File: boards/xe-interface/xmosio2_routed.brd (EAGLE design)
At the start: 116.8 x 55.2 mm, 105 parts, among them IC1 IDTQS3245QSOP20, IC2 IDTQS3245QSOP20, IC3 IDTQS3245QSOP20, IC4 IDTQS3245QSOP20, IC5 IDTQS3245QSOP20, U1 24 MHz Osc. (F535L-24), U2 USD-SOCKETNEW, X1 0446200002

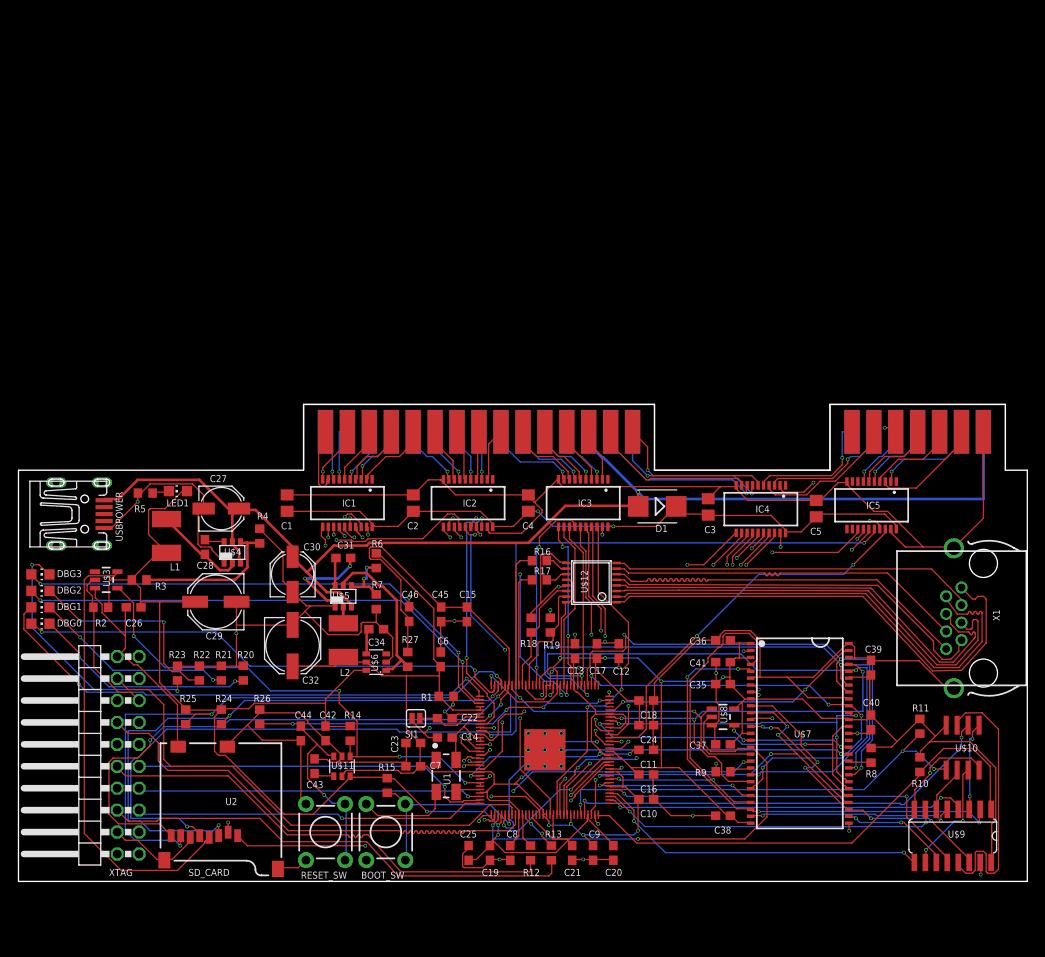
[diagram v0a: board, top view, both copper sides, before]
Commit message: Latest board (routed and unrolled)
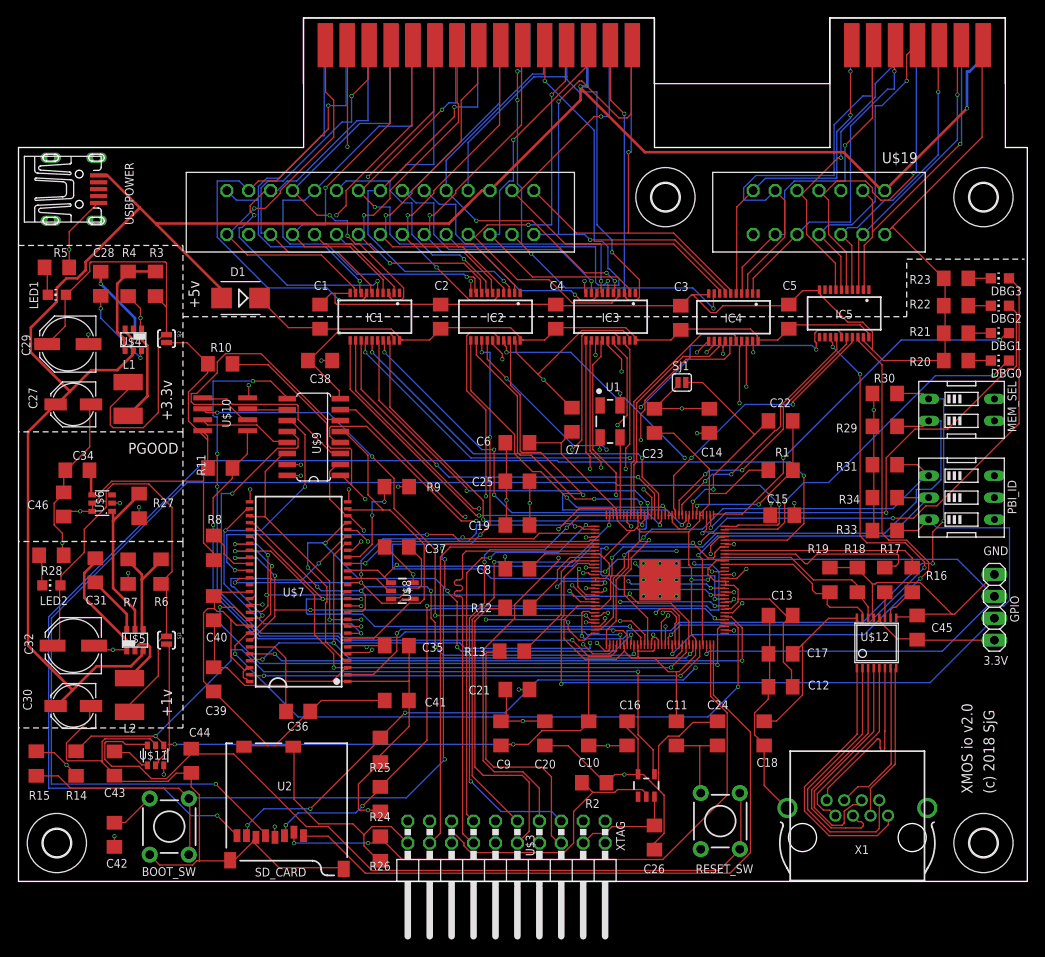
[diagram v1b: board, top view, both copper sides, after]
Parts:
- added GPIO: (no value), pinhead:1X04
- added H1, H2, H3, H4: MOUNT-HOLE3.2, holes:3,2
- added LED2: ok33, led:CHIP-LED0805
- added MEM_SEL: (no value), special:EDG-02
- added PBI_ID: (no value), special:EDG-03
- added R28: 47R, rcl:R1206
- added R29, R30, R31, R33, R34: 10K, rcl:R1206
- added SJ2, SJ3: SOLDERJUMPERNO, SparkFun:SJ_2S-NO
- added U$19: XE_SLOT, pbxl:XE_SLOT
- C1, C2, C3, C4, C5: device rcl:C0805 -> rcl:C1206
- C10, C11, C12, C13, C14, C15, C16, C17, C18, C19, C20, C21, C22, C23, C24, C25, C26, C28, C31, C34, C35, C36, C37, C38, C39, C40, C41, C42, C43, C44, C45, C46, C6, C7, C8, C9: device rcl:C0603 -> rcl:C1206
- R1, R10, R11, R12, R13, R14, R15, R16, R17, R18, R19, R2, R20, R21, R22, R23, R24, R25, R26, R27, R3, R4, R5, R6, R7, R8, R9: device rcl:R0603 -> rcl:R1206
- moved DBG3 116.3 mm to (113.7, 69.8), turned to 90 degrees
- moved DBG2 115.9 mm to (113.7, 66.7), turned to 90 degrees
- moved DBG1 115.6 mm to (113.7, 63.5), turned to 90 degrees
- moved DBG0 115.2 mm to (113.7, 60.3), turned to 90 degrees
- moved R23 101.1 mm to (108.6, 69.8), turned to 180 degrees
- moved R22 97.4 mm to (108.6, 66.7), turned to 180 degrees
- moved R21 93.8 mm to (108.6, 63.5), turned to 180 degrees
- moved U$10 93.7 mm to (23.9, 54.1), turned to 90 degrees
- moved R10 93.4 mm to (23.4, 59.9), turned to 0 degrees
- moved R20 90.1 mm to (108.6, 60.3), turned to 180 degrees
- moved U$9 87.2 mm to (34.2, 51.5), turned to 90 degrees
- moved R11 86.4 mm to (23.4, 47.9), turned to 0 degrees
- moved R8 79.8 mm to (22.6, 38.6), turned to 90 degrees
- moved C40 77.3 mm to (22.6, 31.7), turned to 90 degrees
- moved C39 76.1 mm to (22.6, 23.4), turned to 270 degrees
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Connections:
- new net N$30: C29.+, L1.1, LED1.A, R3.2, SJ2.1
- new net N$31: LED2.C, R28.2
- new net N$32: C32.+, L2.1, LED2.A, R6.2, SJ3.1
- new net N$34: MEM_SEL.2, R29.1, U$2.25
- new net N$35: MEM_SEL.1, R30.2, U$2.26
- new net N$36: GPIO.3, U$2.12
- new net N$37: GPIO.2, U$2.14
- new net PBI0: PBI_ID.1, R31.2, U$2.33
- new net PBI1: PBI_ID.2, R34.2, U$2.61
- new net PBI2: PBI_ID.3, R33.2, U$2.62
- net +5V: now also U$19.26, U$19.44
- net B1: now also U$19.1
- net B10: now also U$19.11
- net B11: now also U$19.12
- net B12: now also U$19.13
- net B13: now also U$19.14
- net B14: now also U$19.15
- net B15: now also U$19.16
- net B16: now also U$19.17
- net B17: now also U$19.18
- net B18: now also U$19.19
- net B19: now also U$19.20
- net B2: now also U$19.2
- net B20: now also U$19.21
- net B21: now also U$19.22
- net B22: now also U$19.23
- net B23: now also U$19.24
- net B24: now also U$19.25
- net B25: now also U$19.27
- net B26: now also U$19.28
- net B27: now also U$19.29
- net B28: now also U$19.30
- net B29: now also U$19.32
- net B3: now also U$19.4
- net B30: now also U$19.33
- net B31: now also U$19.34
- net B32: now also U$19.35
- net B33: now also U$19.36
- net B34: now also U$19.37
- net B35: now also U$19.38
- net B36: now also U$19.39
- net B37: now also U$19.41
- net B38: now also U$19.42
- net B4: now also U$19.5
- net B5: now also U$19.6
- net B6: now also U$19.7
- net B7: now also U$19.8
- net B8: now also U$19.9
- net B9: now also U$19.10
- net GND: now also GPIO.1, R28.1, R29.2, R30.1, R31.1, R33.1, R34.1, U$19.3, U$19.43
- net VCCINT: now also SJ3.2; no longer C32.+, L2.1, R6.2, U$6.5
- net VCCIO: now also GPIO.4, MEM_SEL.3, MEM_SEL.4, PBI_ID.4, PBI_ID.5, PBI_ID.6, SJ2.2, U$6.5; no longer C29.+, L1.1, LED1.A, R3.2
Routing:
- net VCCIO: track 456.0 -> 256.4 mm, vias 10 -> 29
- net +5V: track 145.0 -> 238.6 mm, vias 1 -> 2
- net SDC_D1: track 64.5 -> 155.1 mm
- net GND: track 464.6 -> 551.5 mm, vias 32 -> 37
- net SDC_CLK: track 69.7 -> 147.2 mm
- net N$33: track 23.3 -> 99.8 mm, vias 1 -> 3
- net N$21: track 22.1 -> 96.7 mm, vias 1 -> 0
- net N$35: track 0.00 -> 74.3 mm, vias 0 -> 3
- net N$36: track 0.00 -> 70.2 mm, vias 0 -> 1
- net N$34: track 0.00 -> 62.0 mm, vias 0 -> 1
- net PBI2: track 0.00 -> 61.1 mm, vias 0 -> 1
- net N$32: track 0.00 -> 56.3 mm
- net VCCINT: track 174.3 -> 228.8 mm, vias 10 -> 4
- net PBI0: track 0.00 -> 54.4 mm, vias 0 -> 1
- net N$30: track 0.00 -> 52.6 mm
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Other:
- board size 116.8 x 55.2 mm -> 116.8 x 100 mm
- board text added: "(c) 2018 SjG"
- board text added: "+1v"
- board text added: "+3.3v"
- board text added: "+5v"
- board text added: "3.3V"
- board text added: "GND"
- board text added: "PGOOD"
- board text added: "XMOS io v2.0"
